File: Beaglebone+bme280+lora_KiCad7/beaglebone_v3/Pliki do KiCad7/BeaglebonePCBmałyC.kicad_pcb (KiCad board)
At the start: 2 copper layers, 86.4 x 54.6 mm, 25 parts, among them J2 Screw_Terminal_01x02, J4 Screw_Terminal_01x03, P8 BeagleBone_Black_Header, P9 BeagleBone_Black_Header, U1 RA-02_LORA, U2 ACS725xLCTR-10AU, U3 BME280

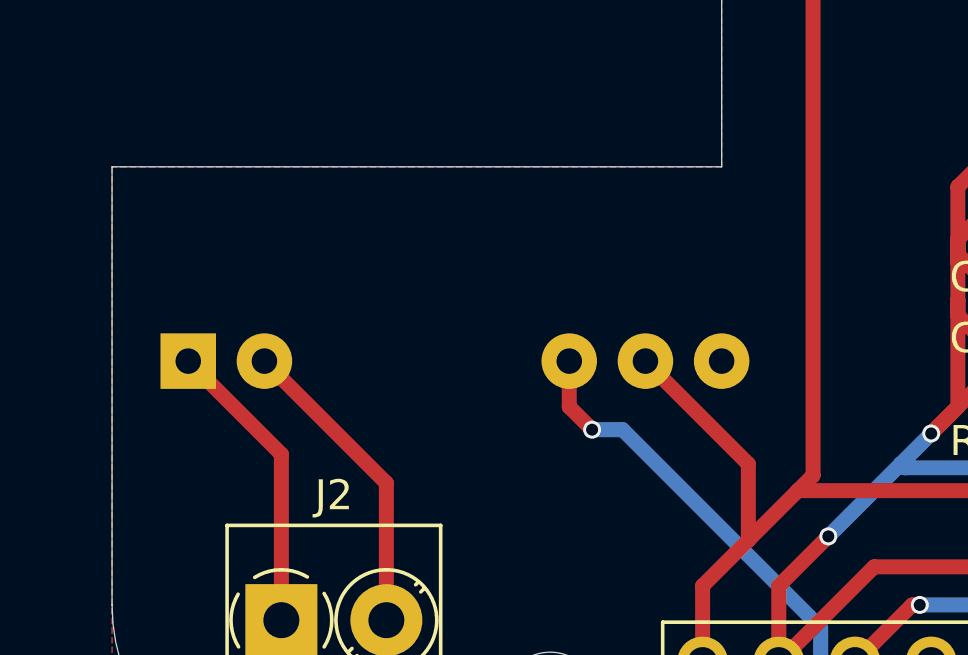
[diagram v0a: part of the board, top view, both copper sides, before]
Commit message: Add files via upload
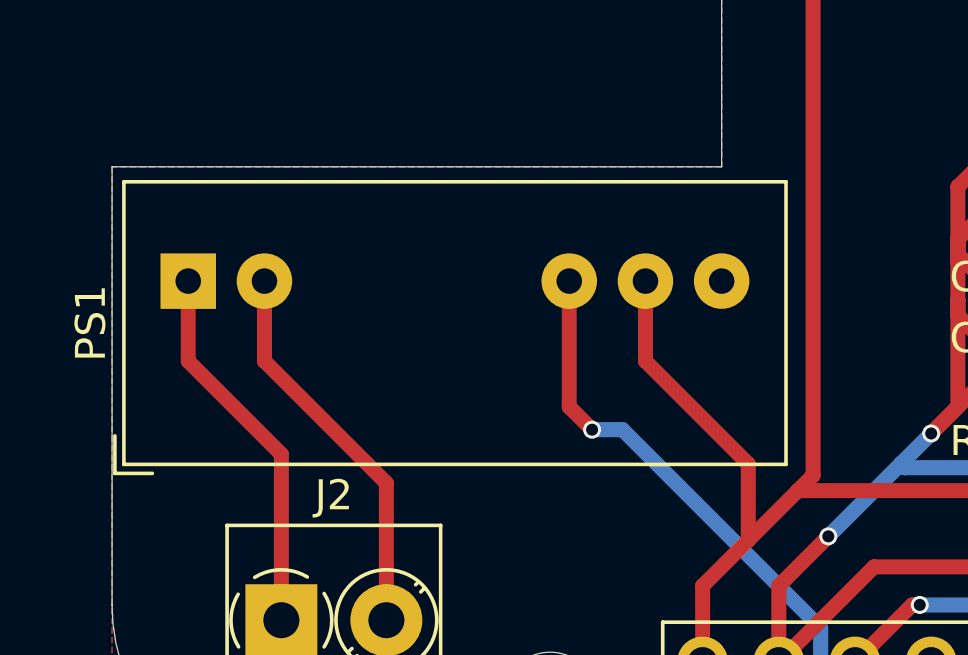
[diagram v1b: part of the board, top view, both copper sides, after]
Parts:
- PS1: moved to F.Cu
- moved PS1 2.67 mm to (102.5, 82.9), turned to 90 degrees
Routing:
- net Net-(J2-Pin_2): track 10.3 -> 13.0 mm
- net Net-(J2-Pin_1): track 9.92 -> 12.6 mm
- net +5V: track 64.5 -> 67.2 mm
- net GNDD: track 141.5 -> 144.1 mm
